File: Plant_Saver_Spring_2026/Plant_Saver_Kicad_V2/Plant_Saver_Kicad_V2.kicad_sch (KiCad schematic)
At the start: 42 parts, among them J1 SBH11-PBPC-D05-ST-BK, J2 SBH11-PBPC-D05-ST-BK, J4 SM04B-SRSS-TB, J5 SM04B-SRSS-TB, J6 Conn_01x02_Pin, J7 Conn_01x06_Socket, J8 25SH-B-03-TR, Q1 G09P02L, Q2 G09P02L, U1 LM66100DCK, U12 LM66100DCK, U2 LM66100DCK, U3 LM66100DCK, U5 ESP32-WROOM-32E-N16

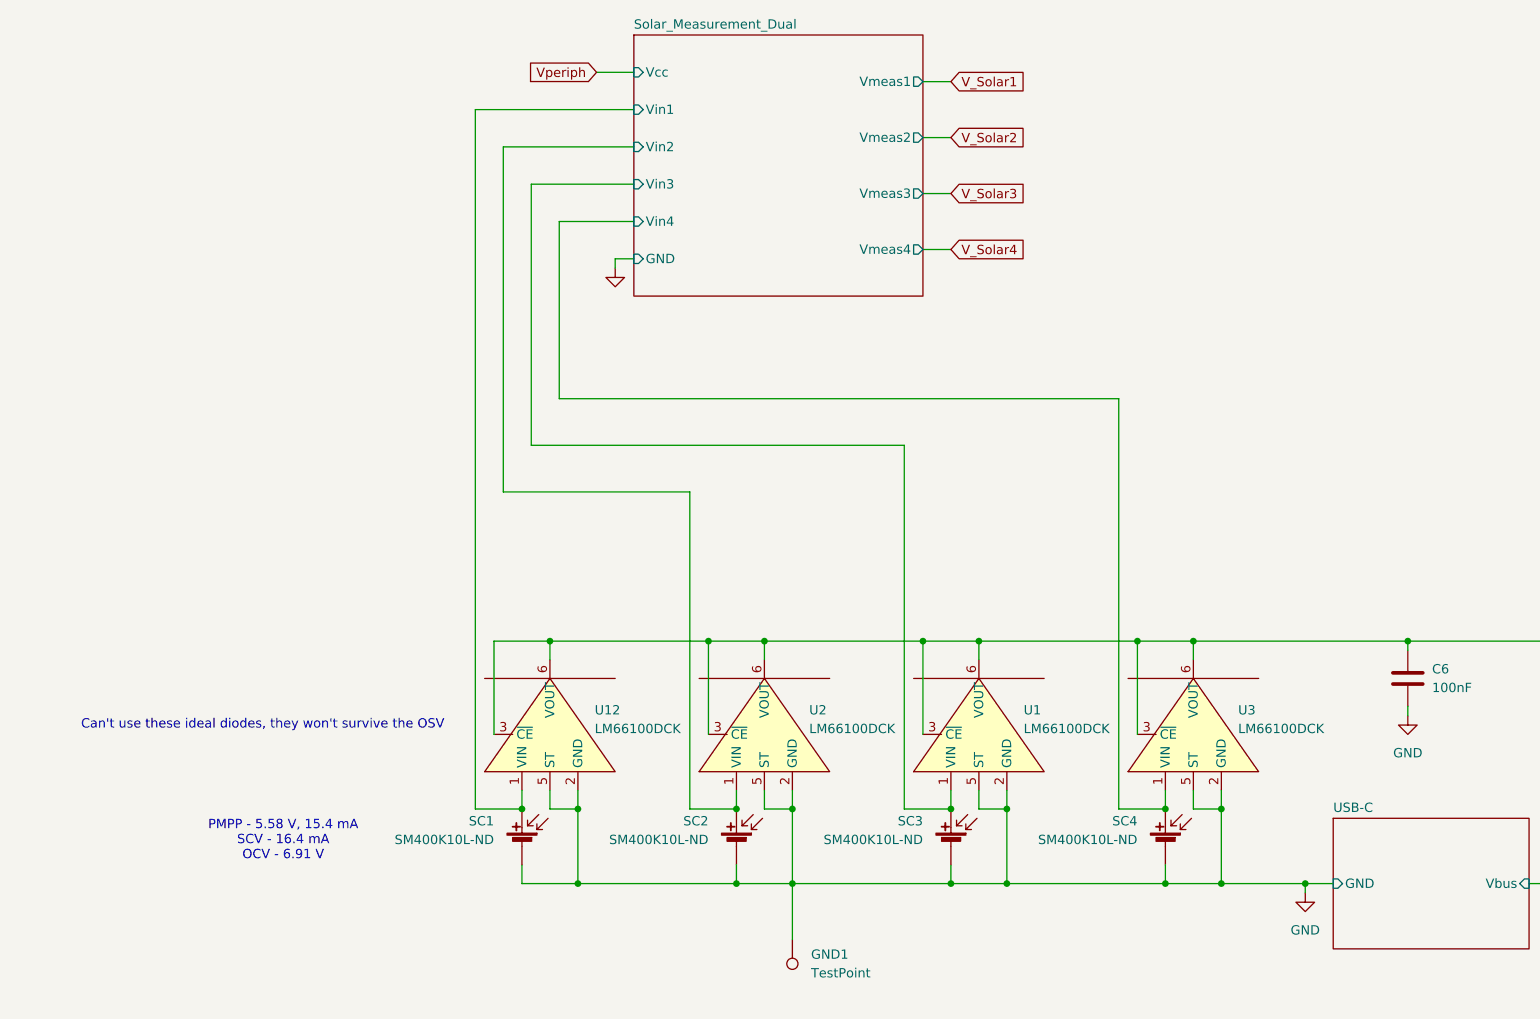
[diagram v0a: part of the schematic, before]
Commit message: Added assets for readme
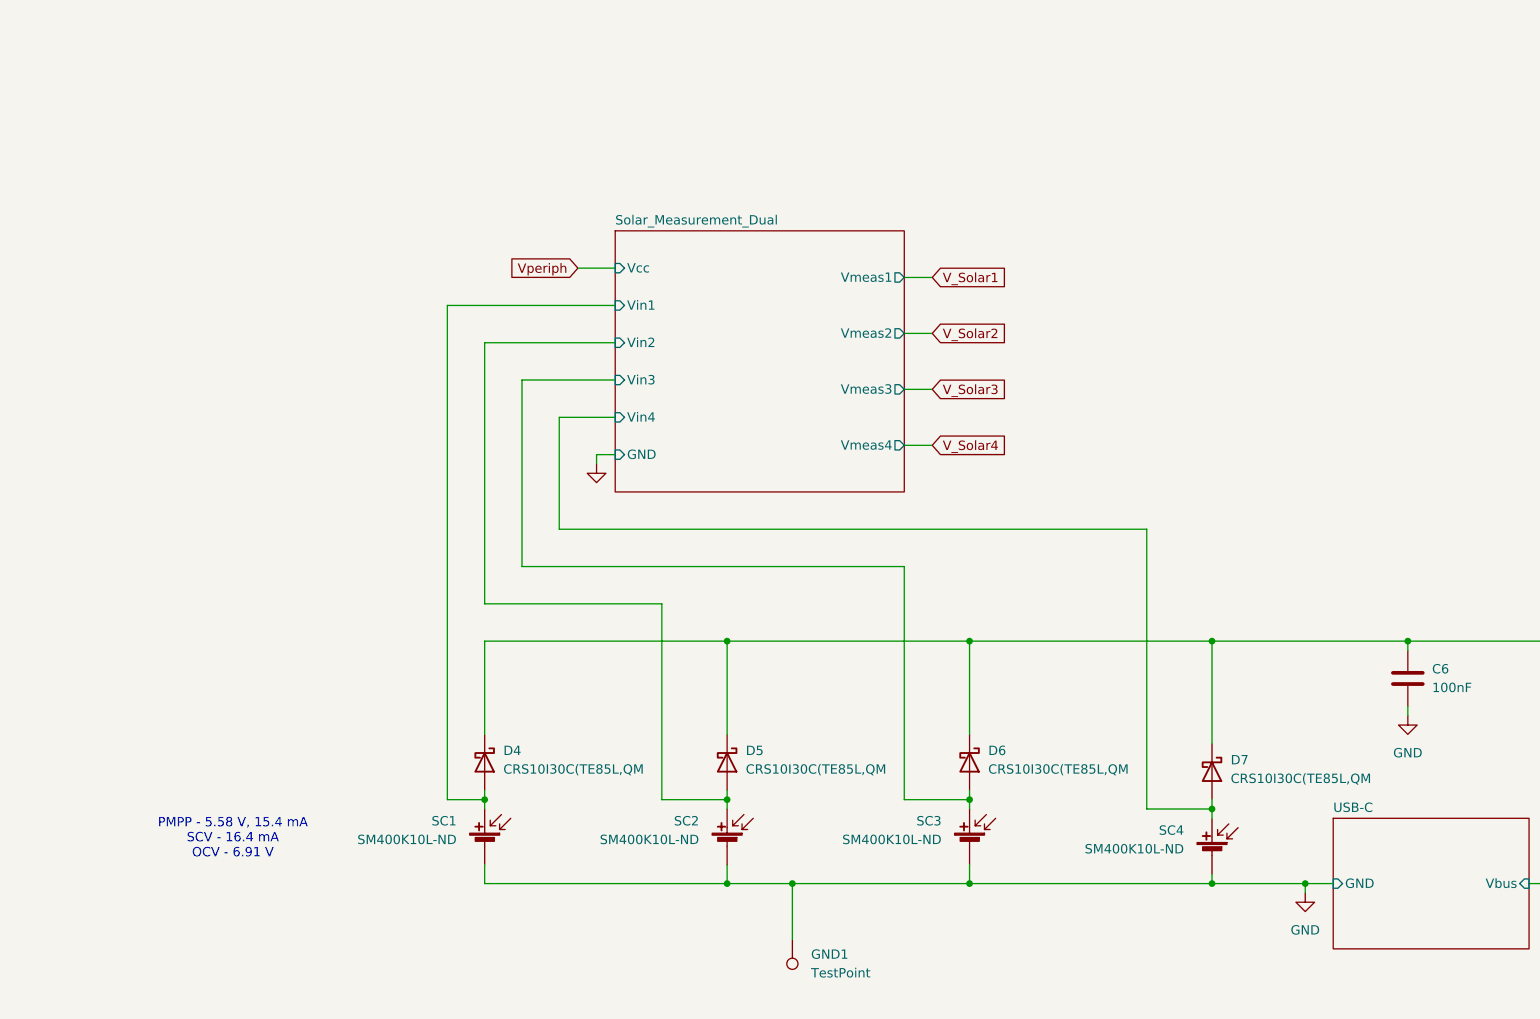
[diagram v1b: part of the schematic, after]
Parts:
- removed U1, U12, U2, U3: LM66100DCK, Package_TO_SOT_SMD:SOT-363_SC-70-6, symbol LM66100DCKR:LM66100DCK
- added D4, D5, D6, D7: CRS10I30C(TE85L,QM, symbol Device:D_Schottky
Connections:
- net Power_And_Charging/Solar: now also D4.1 (K), D5.1 (K), D6.1 (K), D7.1 (K)
- net Solar_Measurement_Dual/Vin1: now also D4.2 (A)
- net Solar_Measurement_Dual/Vin2: now also D5.2 (A)
- net Solar_Measurement_Dual/Vin3: now also D6.2 (A)
- net Solar_Measurement_Dual/Vin4: now also D7.2 (A)
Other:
- note removed: "Can't use these ideal diodes, they won't survive the OSV"
- moved on the sheet: SC1, SC2, SC3, SC4
